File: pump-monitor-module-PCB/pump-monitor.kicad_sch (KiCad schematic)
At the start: 14 parts, among them J1 RJ45_LED, J2 Thermistor_2, J3 SEED C3, J4 CT_jack_input, J5 Thermistor_1, U2 MCP6002-xP

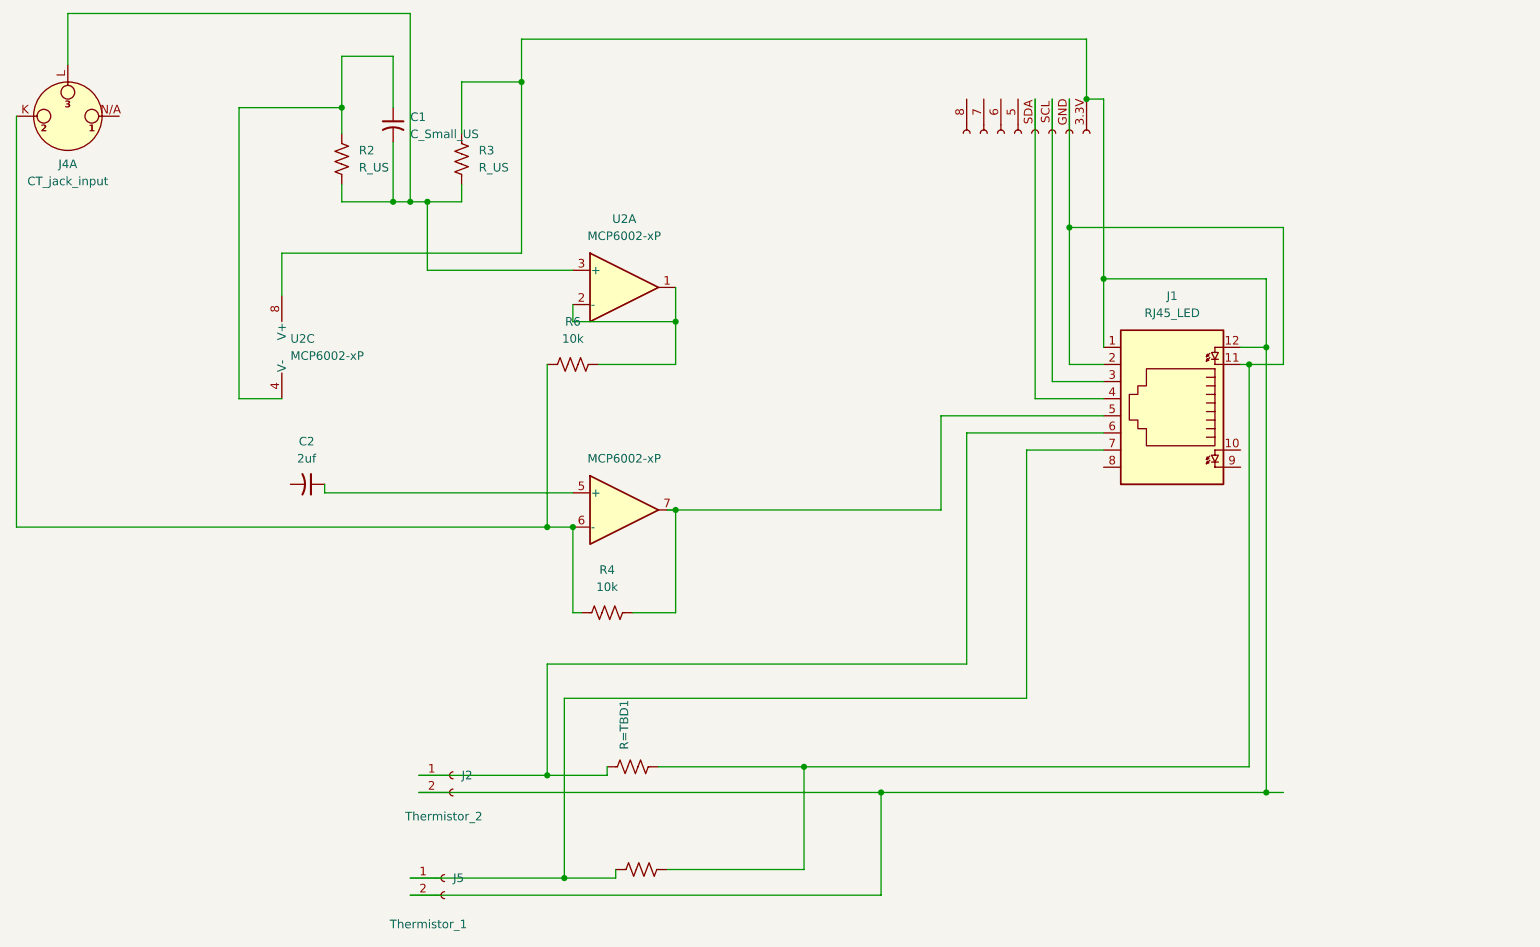
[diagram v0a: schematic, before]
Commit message: trying to migrate
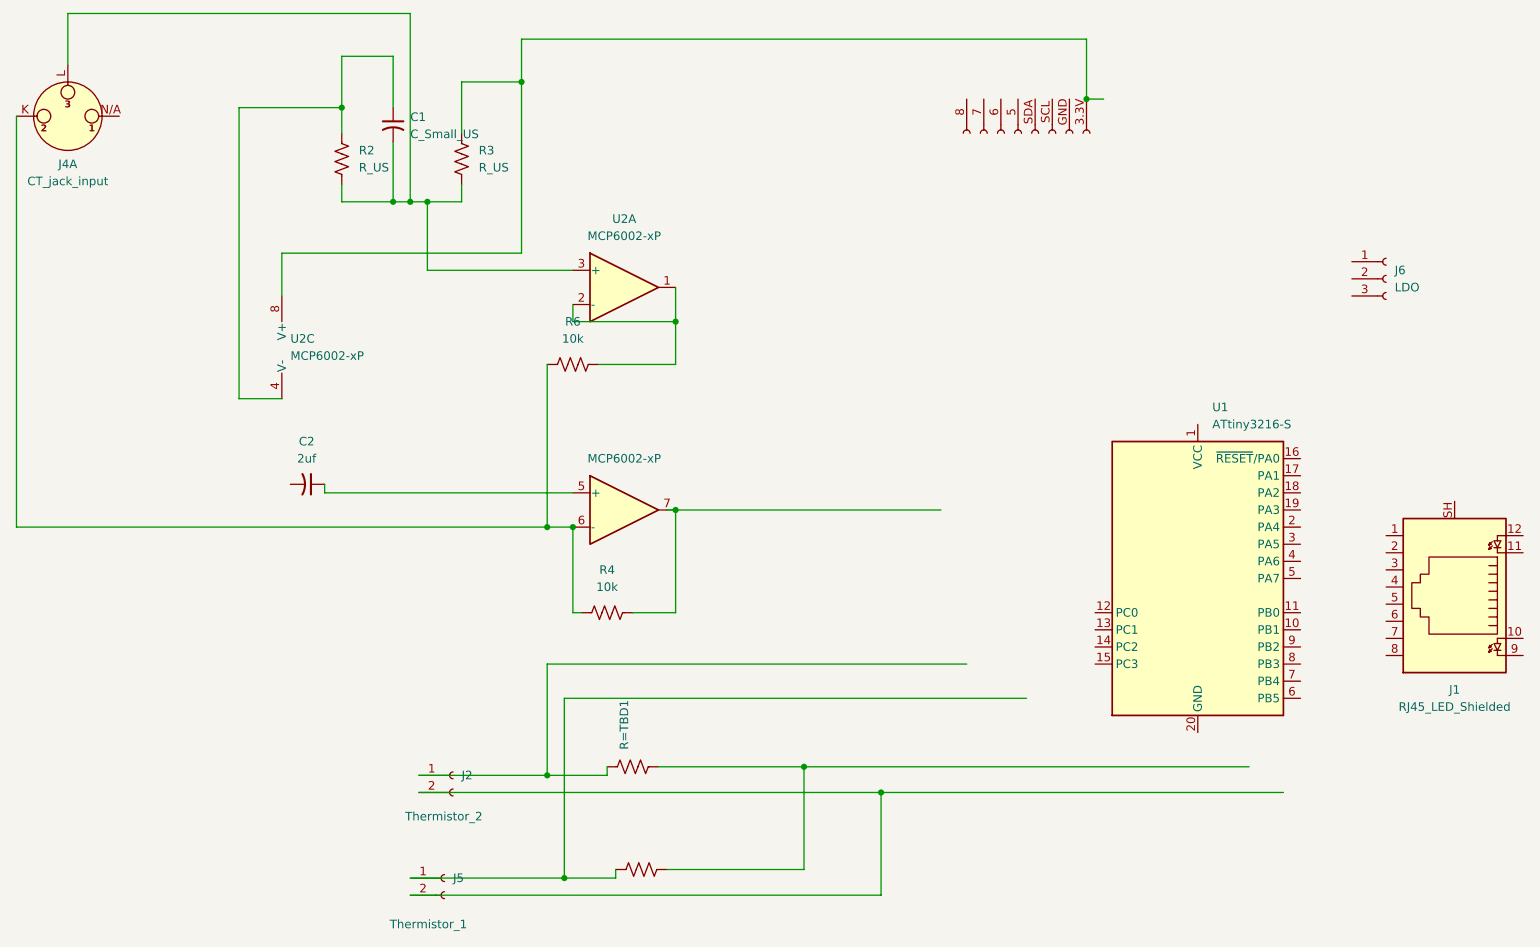
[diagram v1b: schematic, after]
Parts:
- removed J1: RJ45_LED, Connector_RJ:RJ45_Connfly_DS1128-09-S8xx-S_Horizontal, symbol Connector:RJ45_LED
- added J1: RJ45_LED_Shielded, Connector_RJ:RJ45_Amphenol_RJHSE538X, symbol Connector:RJ45_LED_Shielded
- added J6: LDO, symbol Connector:Conn_01x03_Socket
- added U1: ATtiny3216-S, Package_SO:SOIC-20W_7.5x12.8mm_P1.27mm, symbol MCU_Microchip_ATtiny:ATtiny3216-S
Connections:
- net at J3.3.3V (Pin_1), R3.1, U2.8 (V+): no longer J2.2 (Pin_2), J5.2 (Pin_2)
- net at R1.2, R=TBD1.2: no longer J3.GND (Pin_2)
- new net: J2.2 (Pin_2), J5.2 (Pin_2)
